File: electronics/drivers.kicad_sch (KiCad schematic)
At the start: 93 parts, among them J10 Conn_01x05_Pin, J11 Conn_01x01_Pin, J12 Conn_01x01_Pin, J13 Conn_01x02_Pin, J14 Conn_01x02_Pin, J15 VMOT, J16 IOLV / VIO, J17 GND, J18 EXPANSION_HDR, J2 CONT_CFG_DBG, J21 BYPASS_MOTOR_ENABLE, J3 Conn_01x04_Pin, J4 CONT_CFG_DBG, J5 Conn_01x04_Pin, J6 Conn_01x04_Pin, J7 Conn_01x04_Pin, J8 CONT_CFG_DBG, J9 CONT_CFG_DBG, Q3 Q_PMOS, U10 LM1117DT-3.3, U11 74LVC125, U12 ISO7762DBQ, U3 BTT TMC5160 Pro, U4 BTT TMC5160 Pro, U5 BTT TMC5160 Pro, U6 BTT TMC5160 Pro, U8 SFH617A-1, U9 SFH617A-1

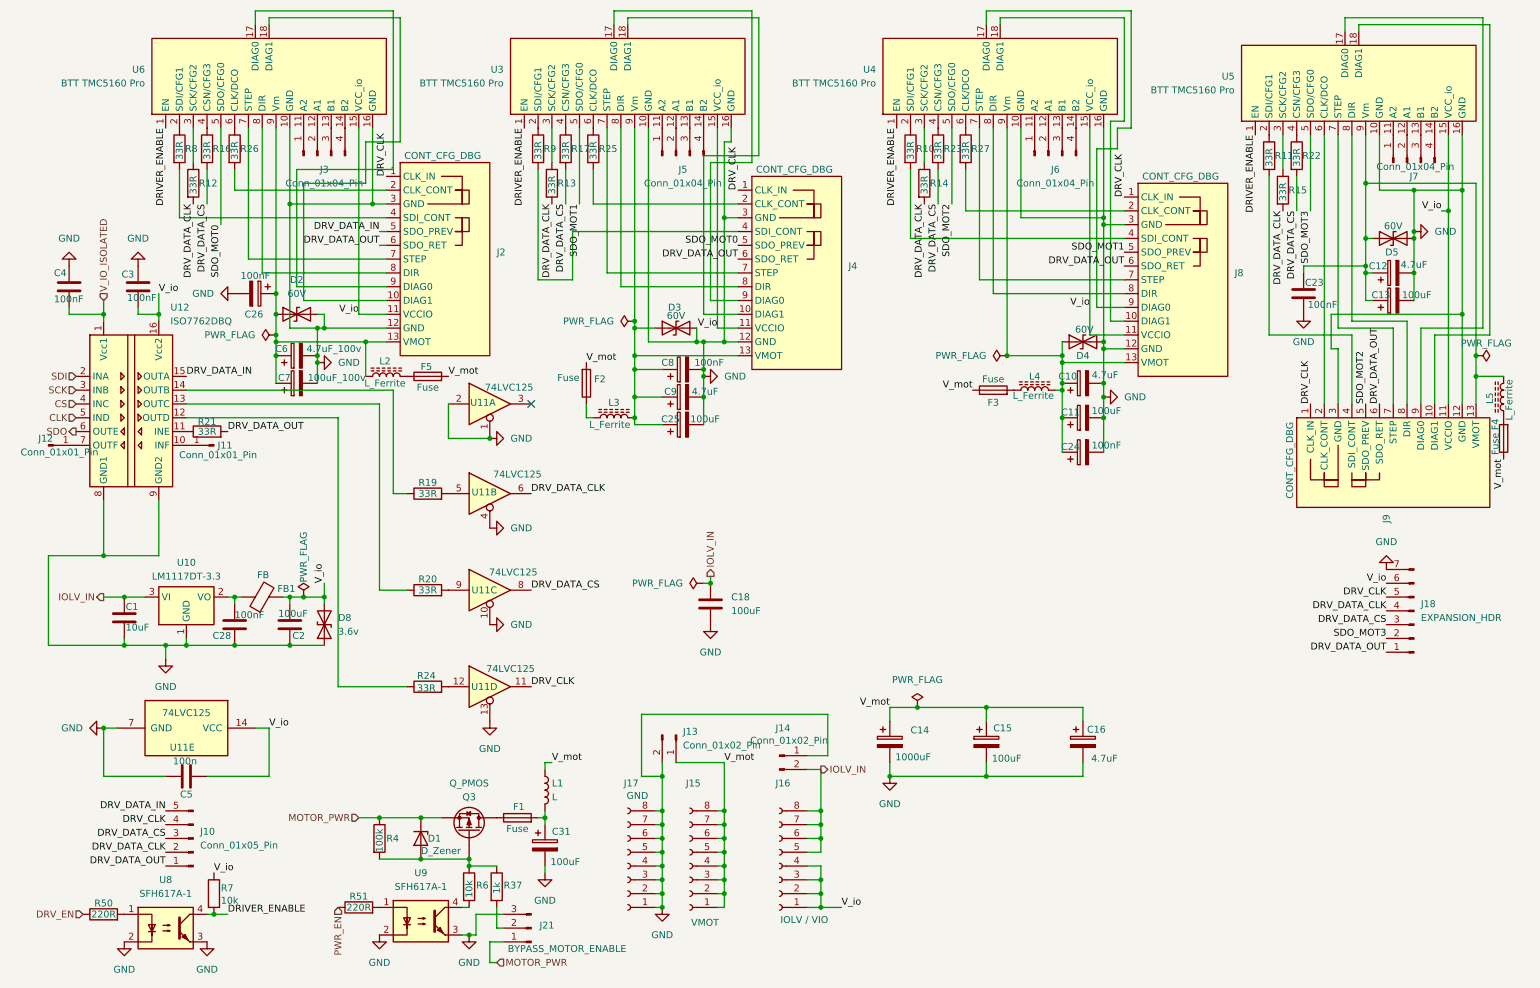
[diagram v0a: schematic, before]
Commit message: saving before i nuke this shit
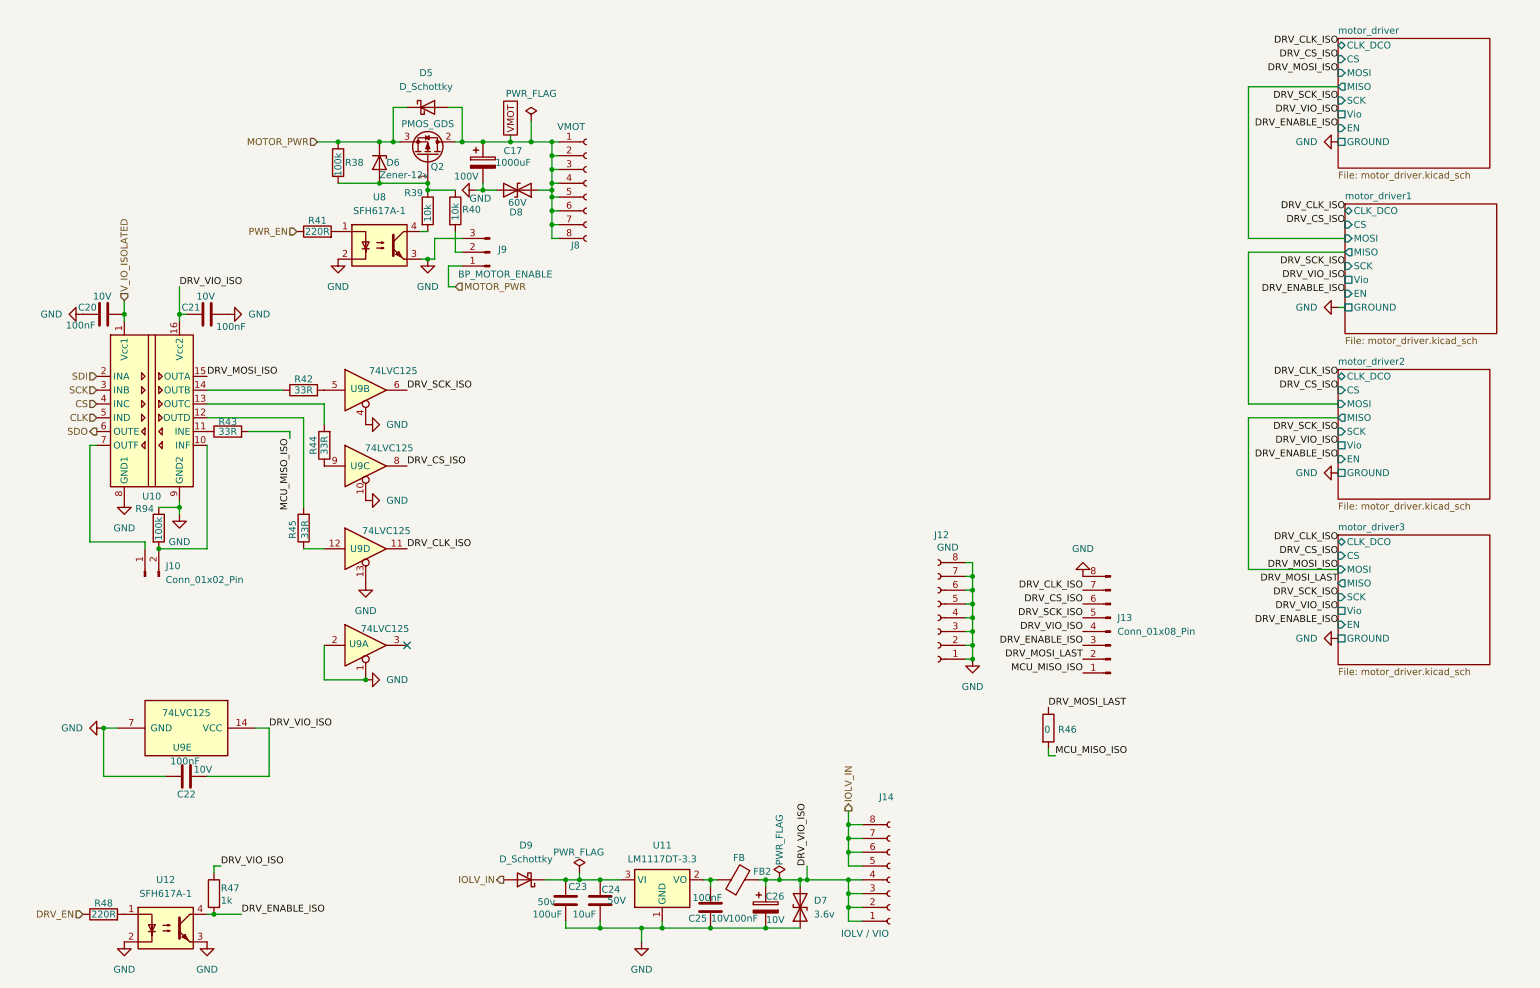
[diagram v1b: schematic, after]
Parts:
- removed C10, C12, C16, C9: 4.7uF, Capacitor_SMD:C_1210_3225Metric_Pad1.33x2.70mm_HandSolder, symbol Device:C_Polarized
- removed C11, C13, C15, C31: 100uF, Capacitor_THT:CP_Radial_D8.0mm_P5.00mm, symbol Device:C_Polarized
- removed C2: 100uF, Capacitor_SMD:C_0805_2012Metric_Pad1.18x1.45mm_HandSolder, symbol Device:C
- removed C23, C4: 100nF, Capacitor_SMD:C_0805_2012Metric_Pad1.18x1.45mm_HandSolder, symbol Device:C
- removed C24, C8: 100nF, Capacitor_SMD:C_0805_2012Metric_Pad1.18x1.45mm_HandSolder, symbol Device:C_Polarized
- removed C25: 100uF, Capacitor_THT:CP_Radial_D6.3mm_P2.50mm, symbol Device:C_Polarized
- removed C6: 4.7uF_100v, Capacitor_SMD:C_1210_3225Metric_Pad1.33x2.70mm_HandSolder, symbol Device:C_Polarized
- removed C7: 100uF_100v, Capacitor_THT:CP_Radial_D8.0mm_P5.00mm, symbol Device:C_Polarized
- removed D2, D3, D4, D5: 60V, symbol Device:D_TVS
- removed F1, F2, F3, F4, F5: Fuse, symbol Device:Fuse
- removed J10: Conn_01x05_Pin, symbol Connector:Conn_01x05_Pin
- removed J11, J12: Conn_01x01_Pin, symbol Connector:Conn_01x01_Pin
- removed J13, J14: Conn_01x02_Pin, symbol Connector:Conn_01x02_Pin
- removed J18: EXPANSION_HDR, symbol Connector:Conn_01x07_Pin
- removed J2, J4, J8, J9: CONT_CFG_DBG, symbol Driver_Motor:CONN_MOTOR
- removed J3, J5, J6, J7: Conn_01x04_Pin, symbol Connector:Conn_01x04_Pin
- removed L1: L, symbol Device:L
- removed L2, L3, L4, L5: L_Ferrite, symbol Device:L_Ferrite
- removed Q3: Q_PMOS, symbol Device:Q_PMOS
- removed R10, R11, R12, R13, R14, R15, R16, R17, R22, R23, R25, R26, R27, R8, R9: 33R, symbol Device:R
- removed U3, U4, U5, U6: BTT TMC5160 Pro, symbol Driver_Motor:BTT-TMC5160-PRO-v1_0
- added C20: 100nF, Capacitor_SMD:C_0805_2012Metric_Pad1.18x1.45mm_HandSolder, symbol Device:C
- added D5, D9: D_Schottky, Diode_THT:D_DO-201AD_P3.81mm_Vertical_AnodeUp, symbol Device:D_Schottky
- added D8: 60V, Diode_THT:D_DO-41_SOD81_P2.54mm_Vertical_AnodeUp, symbol Device:D_TVS
- added J10: Conn_01x02_Pin, Connector_PinSocket_2.54mm:PinSocket_1x02_P2.54mm_Vertical, symbol Connector:Conn_01x02_Pin
- added J13: Conn_01x08_Pin, Connector_PinSocket_2.54mm:PinSocket_1x08_P2.54mm_Vertical, symbol Connector:Conn_01x08_Pin
- added Q2: PMOS_GDS, Package_TO_SOT_THT:TO-220-3_Vertical, symbol Transistor_FET:Q_PMOS_GDS
- added R46: 0, Jumper:SolderJumper-2_P1.3mm_Open_Pad1.0x1.5mm, symbol Device:R
- added R94: 100k, Resistor_SMD:R_0805_2012Metric_Pad1.20x1.40mm_HandSolder, symbol Device:R
- C17: renamed from C14; V (none) -> 100V
- C21: renamed from C3; V (none) -> 10V
- C22: renamed from C5; value 100n -> 100nF; V (none) -> 10V
- C23: renamed from C18; V (none) -> 50v
- C24: renamed from C1; footprint Capacitor_SMD:C_0805_2012Metric_Pad1.18x1.45mm_HandSolder -> Capacitor_THT:CP_Radial_D5.0mm_P2.50mm; V (none) -> 50V
- C25: renamed from C28; V (none) -> 10V
- C26: V (none) -> 10V
- D6: renamed from D1; value D_Zener -> Zener-12v; footprint (none) -> Diode_THT:D_DO-41_SOD81_P2.54mm_Vertical_AnodeUp
- D7: renamed from D8; footprint (none) -> Diode_THT:D_DO-41_SOD81_P2.54mm_Vertical_AnodeUp
- FB2: renamed from FB1; footprint (none) -> Inductor_SMD:L_1210_3225Metric_Pad1.42x2.65mm_HandSolder
- J12: renamed from J17; footprint (none) -> Connector_PinSocket_2.54mm:PinSocket_1x08_P2.54mm_Vertical
- J14: renamed from J16; footprint (none) -> Connector_PinSocket_2.54mm:PinSocket_1x08_P2.54mm_Vertical
- J8: renamed from J15; footprint (none) -> Connector_PinSocket_2.54mm:PinSocket_1x08_P2.54mm_Vertical
- J9: renamed from J21; value BYPASS_MOTOR_ENABLE -> BP_MOTOR_ENABLE; footprint (none) -> Connector_PinSocket_2.54mm:PinSocket_1x03_P2.54mm_Vertical
- R38: renamed from R4; footprint (none) -> Resistor_SMD:R_0805_2012Metric_Pad1.20x1.40mm_HandSolder
- R39: renamed from R6; footprint (none) -> Resistor_SMD:R_0805_2012Metric_Pad1.20x1.40mm_HandSolder
- R40: renamed from R37; value 1k -> 10k; footprint (none) -> Resistor_SMD:R_0805_2012Metric_Pad1.20x1.40mm_HandSolder
- R41: renamed from R51; footprint (none) -> Resistor_THT:R_Axial_DIN0204_L3.6mm_D1.6mm_P1.90mm_Vertical
- R42: renamed from R19; footprint (none) -> Resistor_SMD:R_0805_2012Metric_Pad1.20x1.40mm_HandSolder
- R43: renamed from R21; footprint (none) -> Resistor_SMD:R_0805_2012Metric_Pad1.20x1.40mm_HandSolder
- R44: renamed from R20; footprint (none) -> Resistor_SMD:R_0805_2012Metric_Pad1.20x1.40mm_HandSolder
- R45: renamed from R24; footprint (none) -> Resistor_SMD:R_0805_2012Metric_Pad1.20x1.40mm_HandSolder
- R47: renamed from R7; value 10k -> 1k; footprint (none) -> Resistor_THT:R_Axial_DIN0204_L3.6mm_D1.6mm_P1.90mm_Vertical
- R48: renamed from R50; footprint (none) -> Resistor_THT:R_Axial_DIN0204_L3.6mm_D1.6mm_P1.90mm_Vertical
- U11: renamed from U10; footprint Package_TO_SOT_SMD:TO-252-3_TabPin2 -> Package_TO_SOT_THT:TO-220-3_Vertical
- U9: renamed from U11; footprint (none) -> Package_DIP:DIP-14_W7.62mm
- renumbered U12 to U10, U8 to U12, U9 to U8
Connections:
- net GND: now also C21.2, C20.1, D8.2 (A2), J13.8 (Pin_8), R94.1; no longer C21.1
- net IOLV_IN: now also D9.2 (A); no longer C23.1, C24.1, U11.3 (VI)
- net MOTOR_PWR: now also D5.1 (K), Q2.3 (S)
- net V_IO_ISOLATED: now also C20.2
- net at D6.2 (A), R38.2, R39.1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: now also Q2.1 (G)
- net at U9.9: now also R44.1; no longer R44.2
- net DRV_VIO_ISO: now reaches C26.1
- net DRV_VIO_ISO: now also C21.1, C22.1, D7.2 (A2), FB2.2, J14.1 (Pin_1), J14.2 (Pin_2), J14.3 (Pin_3), J14.4 (Pin_4), R47.1, U10.16 (Vcc2), U9.14 (VCC), J13.4 (Pin_4)
- net at R45.1: now also U9.12; no longer U10.12 (OUTD)
- net at R45.2: now also U10.12 (OUTD); no longer U9.12
- net at U10.13 (OUTC): now also R44.2; no longer R44.1
- net at U10.10 (INF): now also J10.2 (Pin_2), R94.2
- net at U10.7 (OUTF): now also J10.1 (Pin_1)
- net DRIVER_ENABLE renamed DRV_ENABLE_ISO
- net DRV_ENABLE_ISO: now also J13.3 (Pin_3)
- net DRV_CLK renamed DRV_CLK_ISO
- net DRV_CLK_ISO: now also J13.7 (Pin_7)
- net DRV_DATA_CLK renamed DRV_SCK_ISO
- net DRV_SCK_ISO: now also J13.5 (Pin_5)
- net DRV_DATA_CS renamed DRV_CS_ISO
- net DRV_CS_ISO: now also J13.6 (Pin_6)
- net DRV_DATA_IN renamed DRV_MOSI_ISO
- net DRV_DATA_OUT renamed MCU_MISO_ISO
- net MCU_MISO_ISO: now also J13.1 (Pin_1), R46.2
- removed net V_io: C21.2, C22.1, D7.2 (A2), FB2.2, J14.1 (Pin_1), J14.2 (Pin_2), J14.3 (Pin_3), J14.4 (Pin_4), R47.1, U10.16 (Vcc2), U9.14 (VCC)
- net V_mot renamed VMOT
- net VMOT: now also D5.2 (A), D8.1 (A1), Q2.2 (D)
- new net: C23.1, C24.1, D9.1 (K), U11.3 (VI)
- new net DRV_MOSI_LAST: J13.2 (Pin_2), R46.1
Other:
- added sheet motor_driver (motor_driver.kicad_sch)
- added sheet motor_driver1 (motor_driver.kicad_sch)
- added sheet motor_driver2 (motor_driver.kicad_sch)
- added sheet motor_driver3 (motor_driver.kicad_sch)
- moved on the sheet: C17, C21, C23, C24, C25, D6, D7, FB2, J12, J14, J8, J9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
